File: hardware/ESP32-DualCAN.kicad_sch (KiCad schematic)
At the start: 31 parts, among them J1 Molex 70553 6p, J2 Conn_01x10_Socket, J3 Conn_01x10_Socket, J4 holes, J5 pads, J6 holes, J7 pads, U1 LV2862Y, U2 ESP32-C6-SuperMini, U3 TCAN1044AV, U4 TCAN1044AV, U5 ESP32-C6-Zero

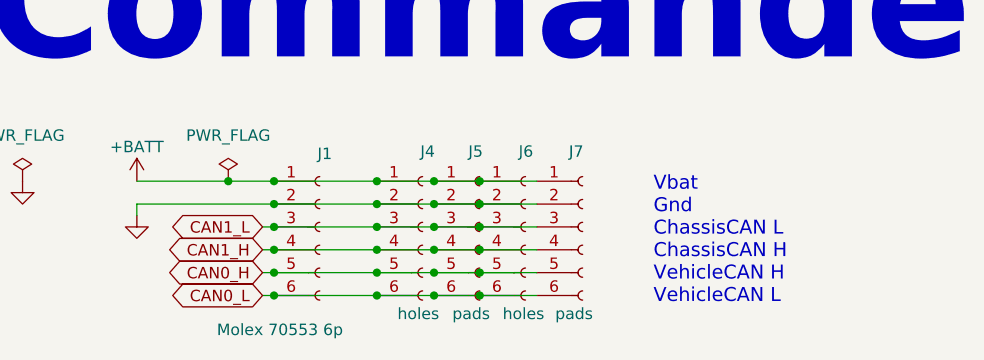
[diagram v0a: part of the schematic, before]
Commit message: kicad 10
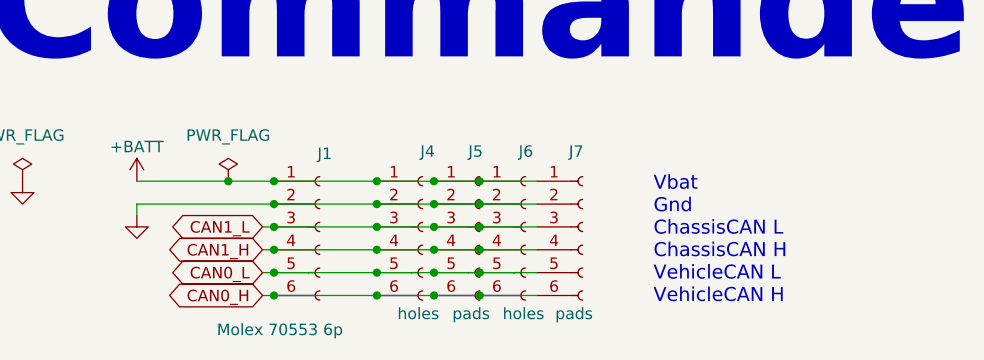
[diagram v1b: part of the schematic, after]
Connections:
- net CAN0_H: now also J1.6 (Pin_6), J4.6 (Pin_6), J5.6 (Pin_6), J6.6 (Pin_6), J7.6 (Pin_6); no longer J1.5 (Pin_5), J4.5 (Pin_5), J5.5 (Pin_5), J6.5 (Pin_5), J7.5 (Pin_5)
- net CAN0_L: now also J1.5 (Pin_5), J4.5 (Pin_5), J5.5 (Pin_5), J6.5 (Pin_5), J7.5 (Pin_5); no longer J1.6 (Pin_6), J4.6 (Pin_6), J5.6 (Pin_6), J6.6 (Pin_6), J7.6 (Pin_6)
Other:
- note added: "Vbat Gnd ChassisCAN L ChassisCAN H VehicleCAN L VehicleCAN H"
- note removed: "Vbat Gnd ChassisCAN L ChassisCAN H VehicleCAN H VehicleCAN L"

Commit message: update pcb
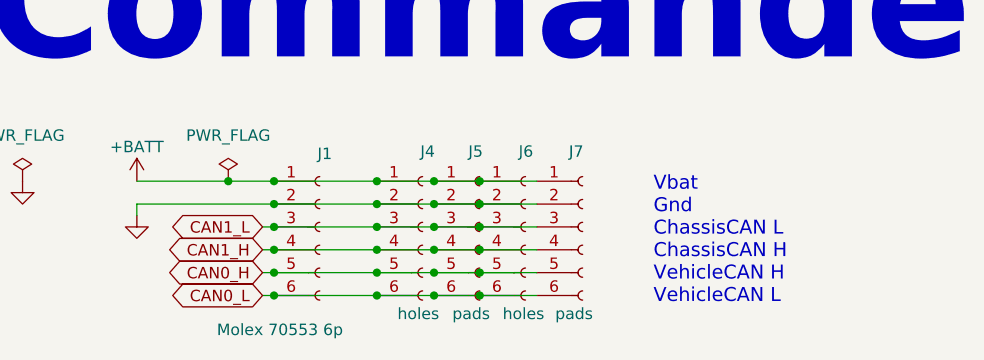
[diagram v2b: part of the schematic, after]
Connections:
- net CAN0_H: now also J1.5 (Pin_5), J4.5 (Pin_5), J5.5 (Pin_5), J6.5 (Pin_5), J7.5 (Pin_5); no longer J1.6 (Pin_6), J4.6 (Pin_6), J5.6 (Pin_6), J6.6 (Pin_6), J7.6 (Pin_6)
- net CAN0_L: now also J1.6 (Pin_6), J4.6 (Pin_6), J5.6 (Pin_6), J6.6 (Pin_6), J7.6 (Pin_6); no longer J1.5 (Pin_5), J4.5 (Pin_5), J5.5 (Pin_5), J6.5 (Pin_5), J7.5 (Pin_5)
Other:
- note added: "Vbat Gnd ChassisCAN L ChassisCAN H VehicleCAN H VehicleCAN L"
- note removed: "Vbat Gnd ChassisCAN L ChassisCAN H VehicleCAN L VehicleCAN H"
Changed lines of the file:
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@@
 		)
 	)
-	(text "Vbat\nGnd\nChassisCAN L\nChassisCAN H\nVehicleCAN L\nVehicleCAN H"
+	(text "Vbat\nGnd\nChassisCAN L\nChassisCAN H\nVehicleCAN H\nVehicleCAN L"
 		(exclude_from_sim no)
 		(at 92.964 185.674 0)
@@
 		)
 	)
-	(global_label "CAN0_L"
+	(global_label "CAN0_H"
 		(shape bidirectional)
 		(at 49.53 189.23 180)
@@
 		)
 		(property "Intersheetrefs" "${INTERSHEET_REFS}"
-			(at 38.5392 189.23 0)
+			(at 38.2368 189.23 0)
 			(hide yes)
 			(show_name no)
@@
 		)
 	)
-	(global_label "CAN0_H"
+	(global_label "CAN0_L"
 		(shape bidirectional)
 		(at 49.53 191.77 180)
@@
 		)
 		(property "Intersheetrefs" "${INTERSHEET_REFS}"
-			(at 38.2368 191.77 0)
+			(at 38.5392 191.77 0)
 			(hide yes)
 			(show_name no)
@@
 		(in_bom no)
 		(on_board yes)
-		(in_pos_files yes)
+		(in_pos_files no)
 		(dnp no)
 		(property "Reference" "J5"
@@
 		(in_bom no)
 		(on_board yes)
-		(in_pos_files yes)
+		(in_pos_files no)
 		(dnp no)
 		(property "Reference" "J6"
@@
 		(in_bom no)
 		(on_board yes)
-		(in_pos_files yes)
+		(in_pos_files no)
 		(dnp no)
 		(property "Reference" "J7"
@@
 		(in_bom no)
 		(on_board yes)
-		(in_pos_files yes)
+		(in_pos_files no)
 		(dnp no)
 		(property "Reference" "J4"
